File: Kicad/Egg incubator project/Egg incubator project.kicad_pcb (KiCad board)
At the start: 2 copper layers, 37 parts, among them J1 AVR-ISP-10, J2 DC 12V, J3 DHT11, J4 HC-05, K1 G5LE-1, M1 Fan, Q1 IRLIZ44N, Q2 2SC1815, SW1 T_UP, SW2 T_DOWN, SW3 RESET, U1 ATmega16A-P, U2 L7805

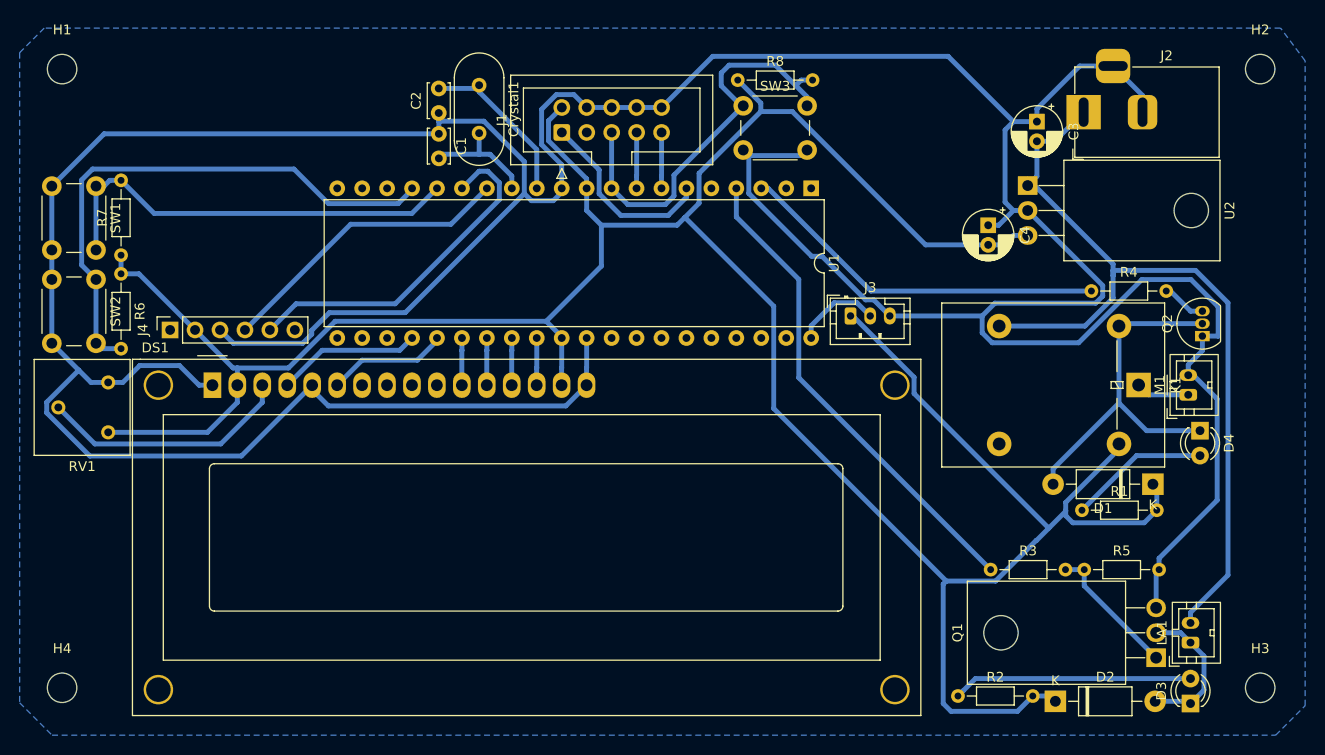
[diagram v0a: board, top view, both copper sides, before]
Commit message: Test file kicad
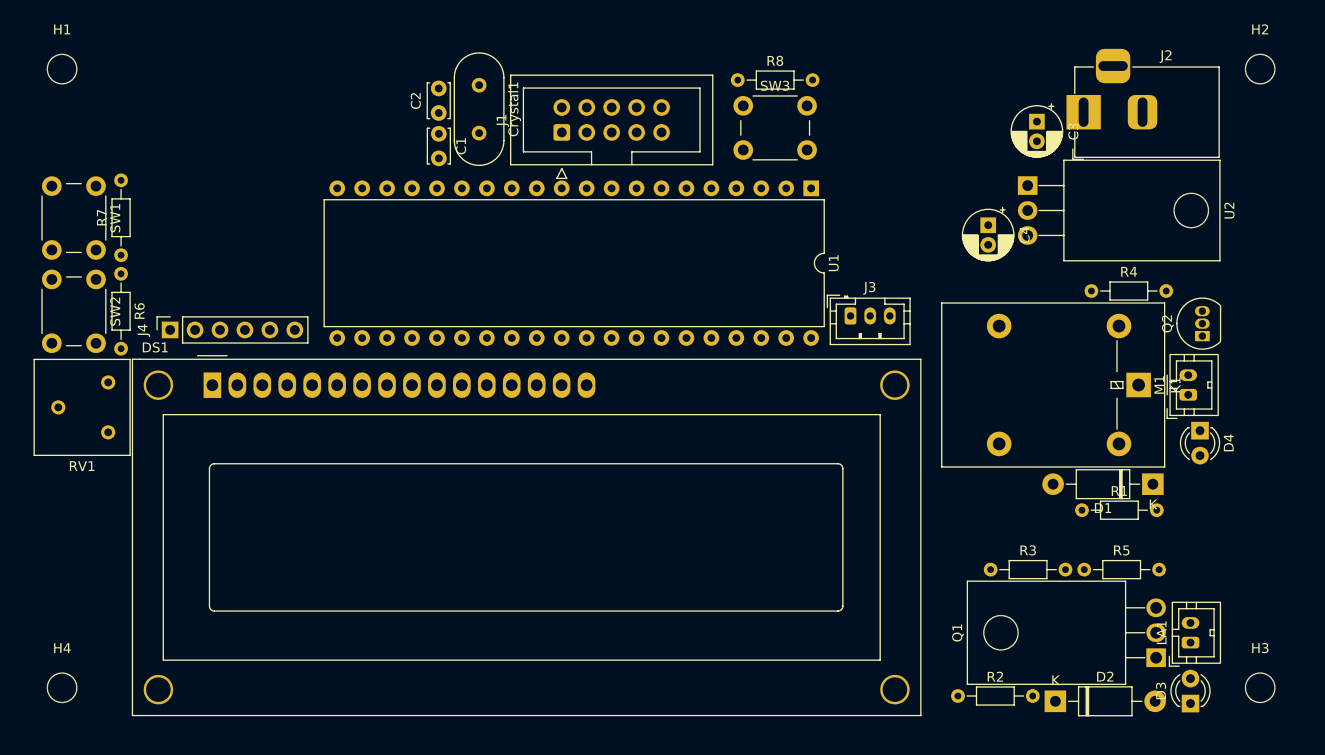
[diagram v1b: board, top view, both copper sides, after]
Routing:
- net GND: track 436.7 -> 0.00 mm
- net 5v: track 304.6 -> 0.00 mm
- net 12v: track 87.7 -> 0.00 mm
- net T_DOWN: track 56.3 -> 0.00 mm
- net LAMP: track 49.6 -> 0.00 mm
- net T_UP: track 43.9 -> 0.00 mm
- net RESET: track 43.5 -> 0.00 mm
- net FAN: track 37.9 -> 0.00 mm
- net Net-(D1-A): track 37.7 -> 0.00 mm
- net TX: track 35.6 -> 0.00 mm
- net RX: track 30.6 -> 0.00 mm
- net Net-(DS1-VO): track 25.8 -> 0.00 mm
- net Net-(D3-A): track 25.2 -> 0.00 mm
- net MOSI: track 19.3 -> 0.00 mm
- net Net-(U1-XTAL2): track 17.0 -> 0.00 mm
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- removed copper zone on B.Cu, net (none)
